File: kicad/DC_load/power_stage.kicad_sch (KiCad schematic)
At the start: 87 parts, among them J2 red_terminal, J3 red terminal, J4 black terminal, J5 black terminal, Q10 MMBT5401, Q11 MMBT5551L, Q12 MMBT5401, Q14 MMBT5551L, Q2 MMBT5401, Q3 FQP19N20C, Q4 FQP19N20C, Q5 FQP19N20C, Q6 FQP19N20C, Q7 MMBT5551L, Q8 MMBT5401, Q9 MMBT5551L, U13 TLV9062, U19 INA181, U20 INA181, U21 INA181, U22 INA181, U5 TLV9062, U6 TLV9062, U7 LMT84LPM

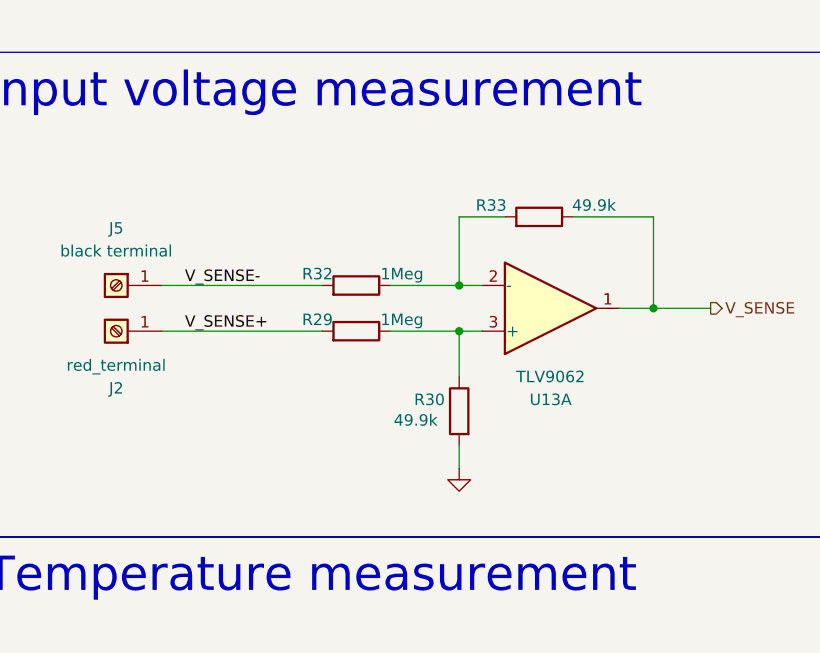
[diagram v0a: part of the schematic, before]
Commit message: Done???.
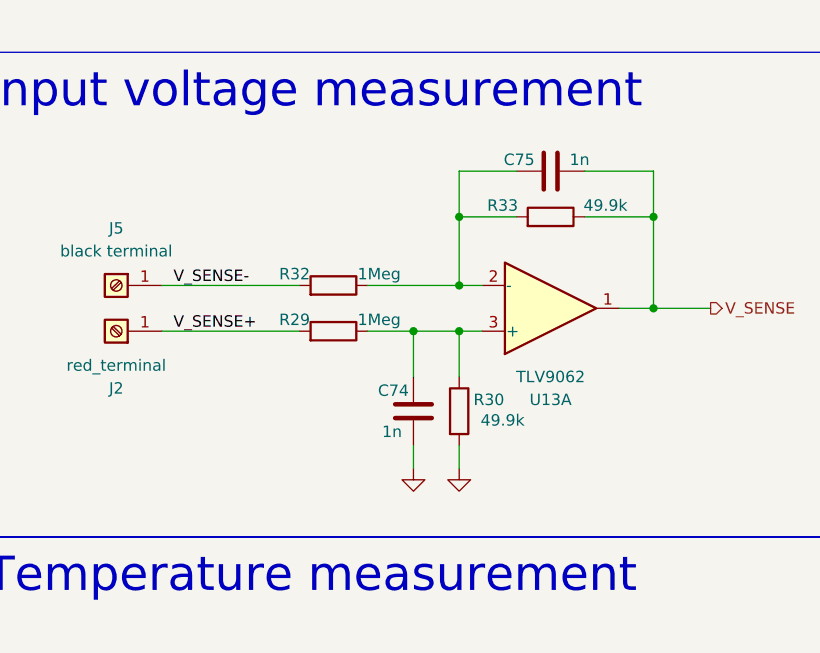
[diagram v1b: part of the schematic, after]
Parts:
- added C74, C75: 1n, Capacitor_SMD:C_0603_1608Metric_Pad1.08x0.95mm_HandSolder, symbol Device:C
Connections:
- net GND: now also C74.1
- net V_SENSE: now also C75.1
- net at R29.1, R30.1, U13.3 (+): now also C74.2
- net at R32.1, R33.2, U13.2 (-): now also C75.2
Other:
- moved on the sheet: R29, R32, R33
